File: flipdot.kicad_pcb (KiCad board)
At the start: 2 copper layers, 121.3 x 14.6 mm, 48 parts, among them J1 Conn_01x02_Pin, J2 Conn_01x02_Pin, J3 Conn_01x02_Pin, J4 Conn_01x12_Pin, U5 74HC595

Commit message: split into separate sheets
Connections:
- net /CLK renamed /row1/CLK
- net /DATA_IN renamed /row1/DATA_IN
- net /DATA_OUT renamed /row1/DATA_OUT
- net /LATCH renamed /row1/LATCH
- net /OE* renamed /row1/OE*

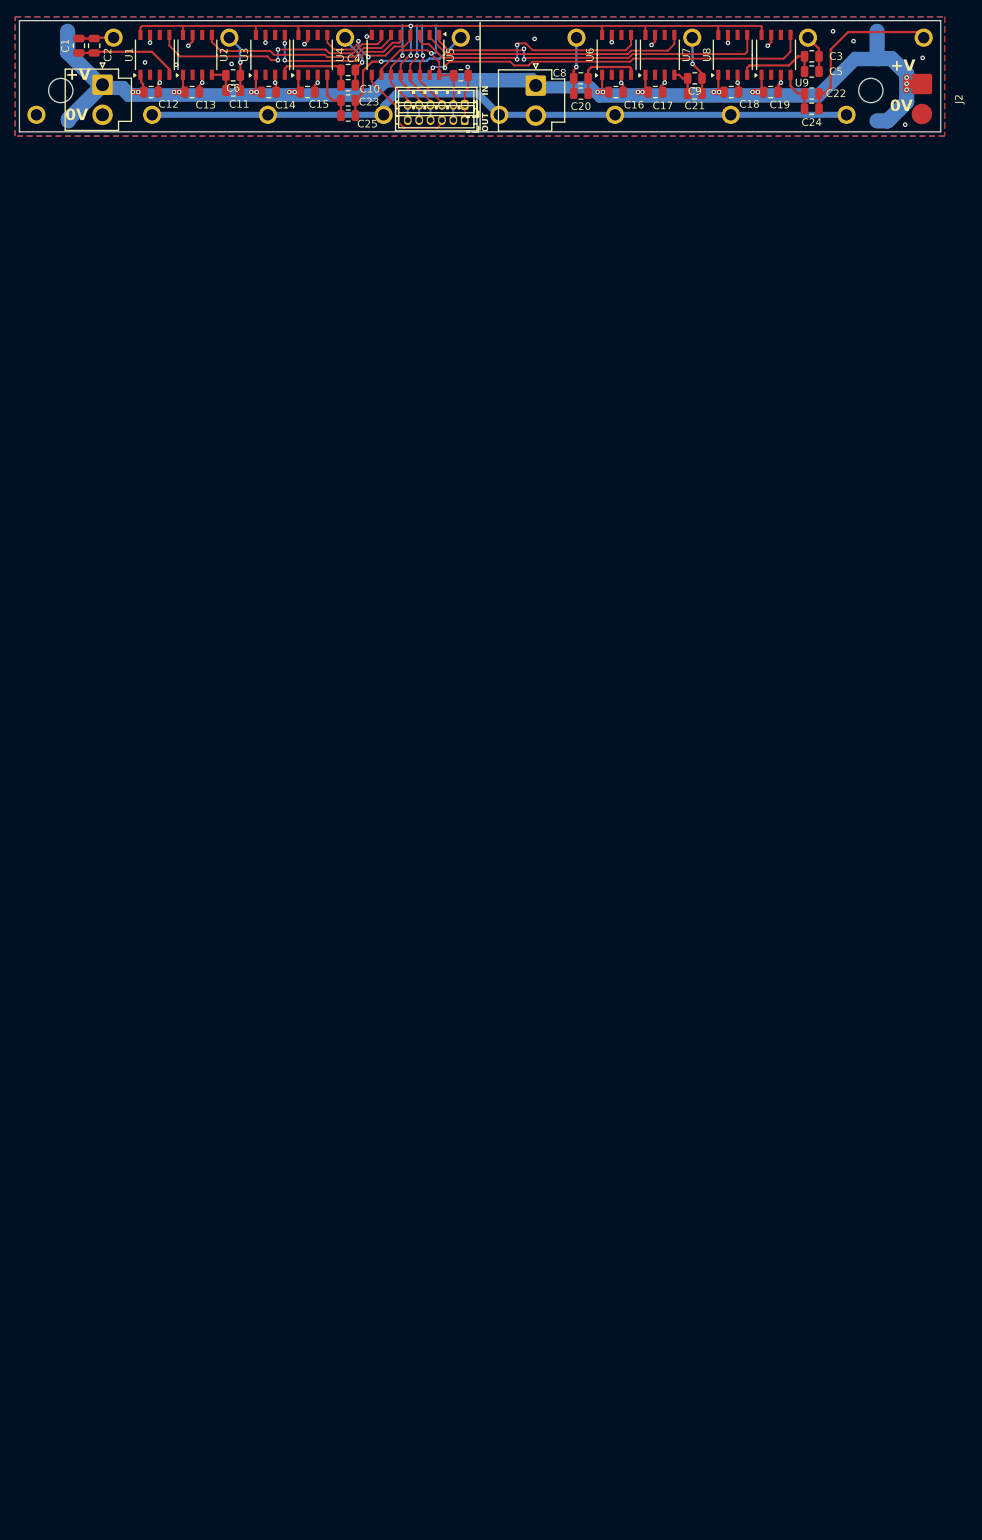
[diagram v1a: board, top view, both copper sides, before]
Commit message: valid 13 row layout
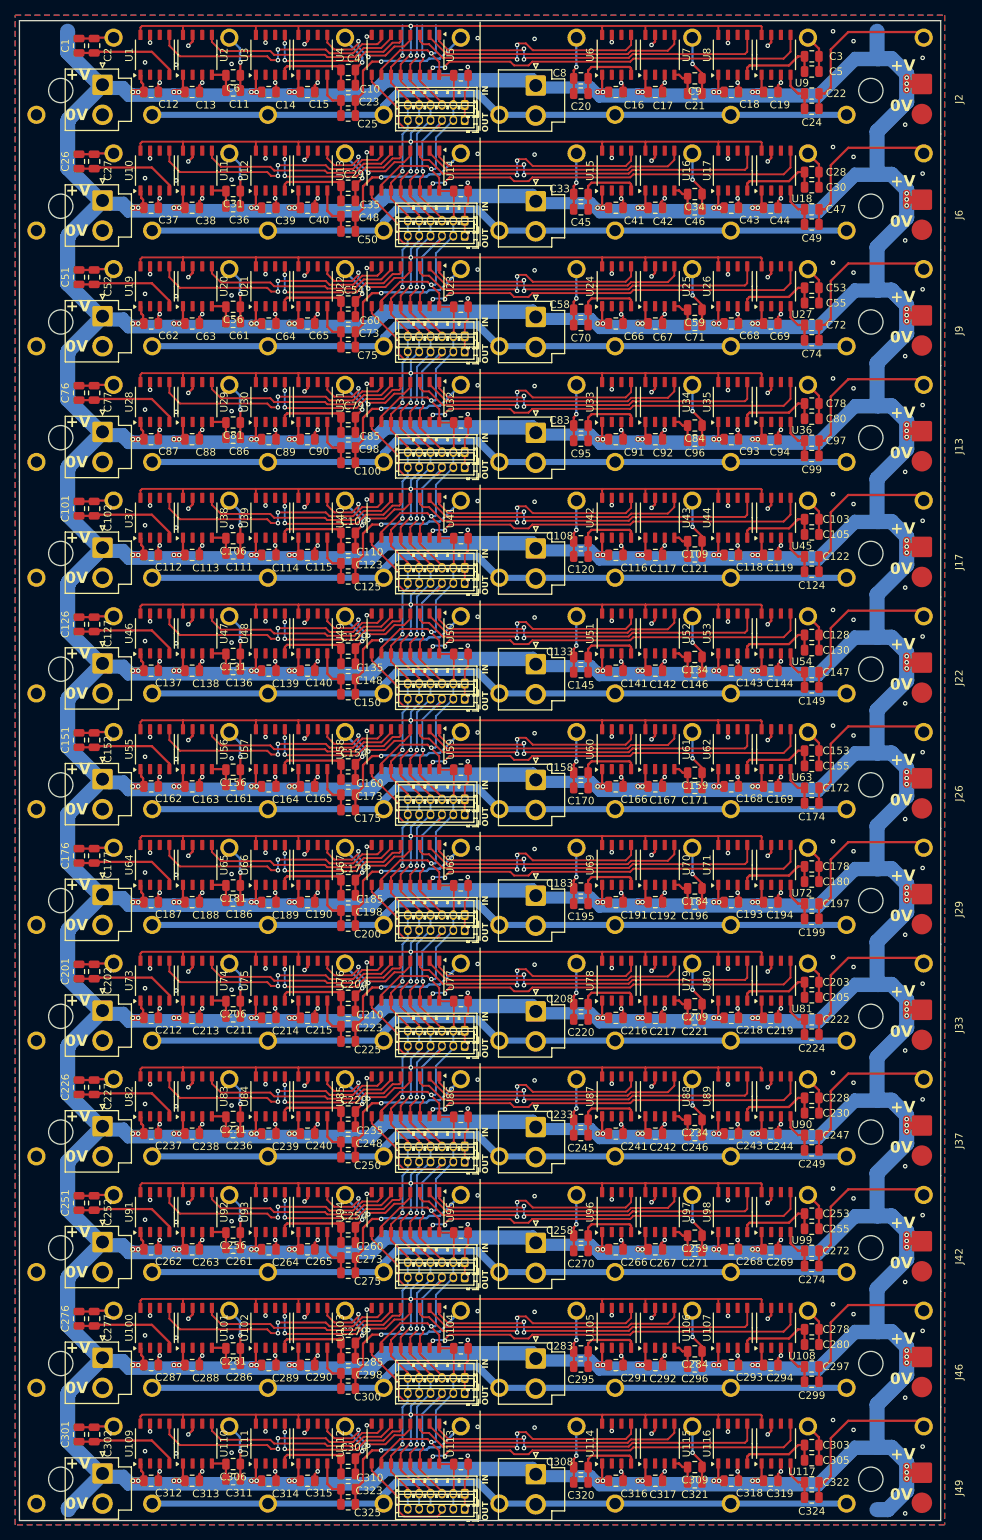
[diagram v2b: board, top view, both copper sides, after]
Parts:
- added C100: 10u, Capacitor_SMD:C_0805_2012Metric, F.Cu at (41.0, 45.8)
- added C101: 10u, Capacitor_SMD:C_0805_2012Metric, F.Cu at (5.60, 51.9)
- added C102: 10u, Capacitor_SMD:C_0805_2012Metric, F.Cu at (7.60, 51.9)
- added C103: 10u, Capacitor_SMD:C_0805_2012Metric, F.Cu at (102.1, 53.3)
- added C104: 10u, Capacitor_SMD:C_0805_2012Metric, F.Cu at (41.0, 55.1)
- added C105: 10u, Capacitor_SMD:C_0805_2012Metric, F.Cu at (102.1, 55.3)
- added C106: 10u, Capacitor_SMD:C_0805_2012Metric, F.Cu at (25.9, 55.8)
- added C107: 10u, Capacitor_SMD:C_0805_2012Metric, F.Cu at (55.9, 55.8)
- added C108: 10u, Capacitor_SMD:C_0805_2012Metric, F.Cu at (71.7, 56.2)
- added C109: 10u, Capacitor_SMD:C_0805_2012Metric, F.Cu at (86.7, 56.2)
- added C110: 10u, Capacitor_SMD:C_0805_2012Metric, F.Cu at (41.0, 57.1)
- added C111: 10u, Capacitor_SMD:C_0805_2012Metric, F.Cu at (25.9, 57.8)
- added C112: 10u, Capacitor_SMD:C_0805_2012Metric, F.Cu at (15.1, 58.0)
- added C113: 10u, Capacitor_SMD:C_0805_2012Metric, F.Cu at (20.5, 58.0)
- added C114: 10u, Capacitor_SMD:C_0805_2012Metric, F.Cu at (30.6, 58.0)
- added C115: 10u, Capacitor_SMD:C_0805_2012Metric, F.Cu at (35.7, 58.0)
- added C116: 10u, Capacitor_SMD:C_0805_2012Metric, F.Cu at (76.3, 58.0)
- added C117: 10u, Capacitor_SMD:C_0805_2012Metric, F.Cu at (81.5, 58.0)
- added C118: 10u, Capacitor_SMD:C_0805_2012Metric, F.Cu at (91.5, 58.0)
- added C119: 10u, Capacitor_SMD:C_0805_2012Metric, F.Cu at (96.7, 58.0)
- added C120: 10u, Capacitor_SMD:C_0805_2012Metric, F.Cu at (71.7, 58.2)
- added C121: 10u, Capacitor_SMD:C_0805_2012Metric, F.Cu at (86.7, 58.2)
- added C122: 10u, Capacitor_SMD:C_0805_2012Metric, F.Cu at (102.1, 58.2)
- added C123: 10u, Capacitor_SMD:C_0805_2012Metric, F.Cu at (41.0, 59.1)
- added C124: 10u, Capacitor_SMD:C_0805_2012Metric, F.Cu at (102.1, 60.2)
- added C125: 10u, Capacitor_SMD:C_0805_2012Metric, F.Cu at (41.0, 61.1)
- added C126: 10u, Capacitor_SMD:C_0805_2012Metric, F.Cu at (5.60, 67.1)
- added C127: 10u, Capacitor_SMD:C_0805_2012Metric, F.Cu at (7.60, 67.1)
- added C128: 10u, Capacitor_SMD:C_0805_2012Metric, F.Cu at (102.1, 68.5)
- added C129: 10u, Capacitor_SMD:C_0805_2012Metric, F.Cu at (41.0, 70.3)
- added C130: 10u, Capacitor_SMD:C_0805_2012Metric, F.Cu at (102.1, 70.5)
- added C131: 10u, Capacitor_SMD:C_0805_2012Metric, F.Cu at (25.9, 71.0)
- added C132: 10u, Capacitor_SMD:C_0805_2012Metric, F.Cu at (55.9, 71.0)
- added C133: 10u, Capacitor_SMD:C_0805_2012Metric, F.Cu at (71.7, 71.4)
- added C134: 10u, Capacitor_SMD:C_0805_2012Metric, F.Cu at (86.7, 71.4)
- added C135: 10u, Capacitor_SMD:C_0805_2012Metric, F.Cu at (41.0, 72.3)
- added C136: 10u, Capacitor_SMD:C_0805_2012Metric, F.Cu at (25.9, 73.0)
- added C137: 10u, Capacitor_SMD:C_0805_2012Metric, F.Cu at (15.1, 73.2)
- added C138: 10u, Capacitor_SMD:C_0805_2012Metric, F.Cu at (20.5, 73.2)
- added C139: 10u, Capacitor_SMD:C_0805_2012Metric, F.Cu at (30.6, 73.2)
- added C140: 10u, Capacitor_SMD:C_0805_2012Metric, F.Cu at (35.7, 73.2)
- added C141: 10u, Capacitor_SMD:C_0805_2012Metric, F.Cu at (76.3, 73.2)
- added C142: 10u, Capacitor_SMD:C_0805_2012Metric, F.Cu at (81.5, 73.2)
- added C143: 10u, Capacitor_SMD:C_0805_2012Metric, F.Cu at (91.5, 73.2)
- added C144: 10u, Capacitor_SMD:C_0805_2012Metric, F.Cu at (96.7, 73.2)
- added C145: 10u, Capacitor_SMD:C_0805_2012Metric, F.Cu at (71.7, 73.4)
- added C146: 10u, Capacitor_SMD:C_0805_2012Metric, F.Cu at (86.7, 73.4)
- added C147: 10u, Capacitor_SMD:C_0805_2012Metric, F.Cu at (102.1, 73.4)
- added C148: 10u, Capacitor_SMD:C_0805_2012Metric, F.Cu at (41.0, 74.3)
- added C149: 10u, Capacitor_SMD:C_0805_2012Metric, F.Cu at (102.1, 75.4)
- added C150: 10u, Capacitor_SMD:C_0805_2012Metric, F.Cu at (41.0, 76.3)
- added C151: 10u, Capacitor_SMD:C_0805_2012Metric, F.Cu at (5.60, 82.3)
- added C152: 10u, Capacitor_SMD:C_0805_2012Metric, F.Cu at (7.60, 82.3)
- added C153: 10u, Capacitor_SMD:C_0805_2012Metric, F.Cu at (102.1, 83.7)
- added C154: 10u, Capacitor_SMD:C_0805_2012Metric, F.Cu at (41.0, 85.5)
- added C155: 10u, Capacitor_SMD:C_0805_2012Metric, F.Cu at (102.1, 85.7)
- added C156: 10u, Capacitor_SMD:C_0805_2012Metric, F.Cu at (25.9, 86.2)
- added C157: 10u, Capacitor_SMD:C_0805_2012Metric, F.Cu at (55.9, 86.2)
- added C158: 10u, Capacitor_SMD:C_0805_2012Metric, F.Cu at (71.7, 86.6)
- added C159: 10u, Capacitor_SMD:C_0805_2012Metric, F.Cu at (86.7, 86.6)
- added C160: 10u, Capacitor_SMD:C_0805_2012Metric, F.Cu at (41.0, 87.5)
- added C161: 10u, Capacitor_SMD:C_0805_2012Metric, F.Cu at (25.9, 88.2)
- added C162: 10u, Capacitor_SMD:C_0805_2012Metric, F.Cu at (15.1, 88.4)
- added C163: 10u, Capacitor_SMD:C_0805_2012Metric, F.Cu at (20.5, 88.4)
- added C164: 10u, Capacitor_SMD:C_0805_2012Metric, F.Cu at (30.6, 88.4)
- added C165: 10u, Capacitor_SMD:C_0805_2012Metric, F.Cu at (35.7, 88.4)
- added C166: 10u, Capacitor_SMD:C_0805_2012Metric, F.Cu at (76.3, 88.4)
- added C167: 10u, Capacitor_SMD:C_0805_2012Metric, F.Cu at (81.5, 88.4)
- added C168: 10u, Capacitor_SMD:C_0805_2012Metric, F.Cu at (91.5, 88.4)
- added C169: 10u, Capacitor_SMD:C_0805_2012Metric, F.Cu at (96.7, 88.4)
- added C170: 10u, Capacitor_SMD:C_0805_2012Metric, F.Cu at (71.7, 88.6)
- added C171: 10u, Capacitor_SMD:C_0805_2012Metric, F.Cu at (86.7, 88.6)
- added C172: 10u, Capacitor_SMD:C_0805_2012Metric, F.Cu at (102.1, 88.6)
- added C173: 10u, Capacitor_SMD:C_0805_2012Metric, F.Cu at (41.0, 89.5)
- added C174: 10u, Capacitor_SMD:C_0805_2012Metric, F.Cu at (102.1, 90.6)
- added C175: 10u, Capacitor_SMD:C_0805_2012Metric, F.Cu at (41.0, 91.5)
- added C176: 10u, Capacitor_SMD:C_0805_2012Metric, F.Cu at (5.60, 97.6)
- added C177: 10u, Capacitor_SMD:C_0805_2012Metric, F.Cu at (7.60, 97.6)
- added C178: 10u, Capacitor_SMD:C_0805_2012Metric, F.Cu at (102.1, 99.0)
- added C179: 10u, Capacitor_SMD:C_0805_2012Metric, F.Cu at (41.0, 100.8)
- added C180: 10u, Capacitor_SMD:C_0805_2012Metric, F.Cu at (102.1, 101.0)
- added C181: 10u, Capacitor_SMD:C_0805_2012Metric, F.Cu at (25.9, 101.5)
- added C182: 10u, Capacitor_SMD:C_0805_2012Metric, F.Cu at (55.9, 101.5)
- added C183: 10u, Capacitor_SMD:C_0805_2012Metric, F.Cu at (71.7, 101.9)
- added C184: 10u, Capacitor_SMD:C_0805_2012Metric, F.Cu at (86.7, 101.9)
- added C185: 10u, Capacitor_SMD:C_0805_2012Metric, F.Cu at (41.0, 102.8)
- added C186: 10u, Capacitor_SMD:C_0805_2012Metric, F.Cu at (25.9, 103.5)
- added C187: 10u, Capacitor_SMD:C_0805_2012Metric, F.Cu at (15.1, 103.7)
- added C188: 10u, Capacitor_SMD:C_0805_2012Metric, F.Cu at (20.5, 103.7)
- added C189: 10u, Capacitor_SMD:C_0805_2012Metric, F.Cu at (30.6, 103.7)
- added C190: 10u, Capacitor_SMD:C_0805_2012Metric, F.Cu at (35.7, 103.7)
- added C191: 10u, Capacitor_SMD:C_0805_2012Metric, F.Cu at (76.3, 103.7)
- added C192: 10u, Capacitor_SMD:C_0805_2012Metric, F.Cu at (81.5, 103.7)
- added C193: 10u, Capacitor_SMD:C_0805_2012Metric, F.Cu at (91.5, 103.7)
- added C194: 10u, Capacitor_SMD:C_0805_2012Metric, F.Cu at (96.7, 103.7)
- added C195: 10u, Capacitor_SMD:C_0805_2012Metric, F.Cu at (71.7, 103.9)
- added C196: 10u, Capacitor_SMD:C_0805_2012Metric, F.Cu at (86.7, 103.9)
- added C197: 10u, Capacitor_SMD:C_0805_2012Metric, F.Cu at (102.1, 103.9)
- added C198: 10u, Capacitor_SMD:C_0805_2012Metric, F.Cu at (41.0, 104.8)
- added C199: 10u, Capacitor_SMD:C_0805_2012Metric, F.Cu at (102.1, 105.9)
- added C200: 10u, Capacitor_SMD:C_0805_2012Metric, F.Cu at (41.0, 106.8)
- added C201: 10u, Capacitor_SMD:C_0805_2012Metric, F.Cu at (5.60, 112.8)
- added C202: 10u, Capacitor_SMD:C_0805_2012Metric, F.Cu at (7.60, 112.8)
- added C203: 10u, Capacitor_SMD:C_0805_2012Metric, F.Cu at (102.1, 114.2)
- added C204: 10u, Capacitor_SMD:C_0805_2012Metric, F.Cu at (41.0, 116.0)
- added C205: 10u, Capacitor_SMD:C_0805_2012Metric, F.Cu at (102.1, 116.2)
- added C206: 10u, Capacitor_SMD:C_0805_2012Metric, F.Cu at (25.9, 116.7)
- added C207: 10u, Capacitor_SMD:C_0805_2012Metric, F.Cu at (55.9, 116.7)
- added C208: 10u, Capacitor_SMD:C_0805_2012Metric, F.Cu at (71.7, 117.1)
- added C209: 10u, Capacitor_SMD:C_0805_2012Metric, F.Cu at (86.7, 117.1)
- added C210: 10u, Capacitor_SMD:C_0805_2012Metric, F.Cu at (41.0, 118.0)
- added C211: 10u, Capacitor_SMD:C_0805_2012Metric, F.Cu at (25.9, 118.7)
- added C212: 10u, Capacitor_SMD:C_0805_2012Metric, F.Cu at (15.1, 118.9)
- added C213: 10u, Capacitor_SMD:C_0805_2012Metric, F.Cu at (20.5, 118.9)
- added C214: 10u, Capacitor_SMD:C_0805_2012Metric, F.Cu at (30.6, 118.9)
- added C215: 10u, Capacitor_SMD:C_0805_2012Metric, F.Cu at (35.7, 118.9)
- added C216: 10u, Capacitor_SMD:C_0805_2012Metric, F.Cu at (76.3, 118.9)
- added C217: 10u, Capacitor_SMD:C_0805_2012Metric, F.Cu at (81.5, 118.9)
- added C218: 10u, Capacitor_SMD:C_0805_2012Metric, F.Cu at (91.5, 118.9)
- added C219: 10u, Capacitor_SMD:C_0805_2012Metric, F.Cu at (96.7, 118.9)
- added C220: 10u, Capacitor_SMD:C_0805_2012Metric, F.Cu at (71.7, 119.1)
- added C221: 10u, Capacitor_SMD:C_0805_2012Metric, F.Cu at (86.7, 119.1)
- added C222: 10u, Capacitor_SMD:C_0805_2012Metric, F.Cu at (102.1, 119.1)
- added C223: 10u, Capacitor_SMD:C_0805_2012Metric, F.Cu at (41.0, 120.0)
- added C224: 10u, Capacitor_SMD:C_0805_2012Metric, F.Cu at (102.1, 121.1)
- added C225: 10u, Capacitor_SMD:C_0805_2012Metric, F.Cu at (41.0, 122.0)
- added C226: 10u, Capacitor_SMD:C_0805_2012Metric, F.Cu at (5.60, 128.1)
- added C227: 10u, Capacitor_SMD:C_0805_2012Metric, F.Cu at (7.60, 128.1)
- added C228: 10u, Capacitor_SMD:C_0805_2012Metric, F.Cu at (102.1, 129.5)
- added C229: 10u, Capacitor_SMD:C_0805_2012Metric, F.Cu at (41.0, 131.3)
- added C230: 10u, Capacitor_SMD:C_0805_2012Metric, F.Cu at (102.1, 131.5)
- added C231: 10u, Capacitor_SMD:C_0805_2012Metric, F.Cu at (25.9, 132.0)
- added C232: 10u, Capacitor_SMD:C_0805_2012Metric, F.Cu at (55.9, 132.0)
- added C233: 10u, Capacitor_SMD:C_0805_2012Metric, F.Cu at (71.7, 132.4)
- added C234: 10u, Capacitor_SMD:C_0805_2012Metric, F.Cu at (86.7, 132.4)
- added C235: 10u, Capacitor_SMD:C_0805_2012Metric, F.Cu at (41.0, 133.3)
- added C236: 10u, Capacitor_SMD:C_0805_2012Metric, F.Cu at (25.9, 134.0)
- added C237: 10u, Capacitor_SMD:C_0805_2012Metric, F.Cu at (15.1, 134.2)
- added C238: 10u, Capacitor_SMD:C_0805_2012Metric, F.Cu at (20.5, 134.2)
- added C239: 10u, Capacitor_SMD:C_0805_2012Metric, F.Cu at (30.6, 134.2)
- added C240: 10u, Capacitor_SMD:C_0805_2012Metric, F.Cu at (35.7, 134.2)
- added C241: 10u, Capacitor_SMD:C_0805_2012Metric, F.Cu at (76.3, 134.2)
- added C242: 10u, Capacitor_SMD:C_0805_2012Metric, F.Cu at (81.5, 134.2)
- added C243: 10u, Capacitor_SMD:C_0805_2012Metric, F.Cu at (91.5, 134.2)
- added C244: 10u, Capacitor_SMD:C_0805_2012Metric, F.Cu at (96.7, 134.2)
- added C245: 10u, Capacitor_SMD:C_0805_2012Metric, F.Cu at (71.7, 134.4)
- added C246: 10u, Capacitor_SMD:C_0805_2012Metric, F.Cu at (86.7, 134.4)
- added C247: 10u, Capacitor_SMD:C_0805_2012Metric, F.Cu at (102.1, 134.4)
- added C248: 10u, Capacitor_SMD:C_0805_2012Metric, F.Cu at (41.0, 135.3)
- added C249: 10u, Capacitor_SMD:C_0805_2012Metric, F.Cu at (102.1, 136.4)
- added C250: 10u, Capacitor_SMD:C_0805_2012Metric, F.Cu at (41.0, 137.3)
- added C251: 10u, Capacitor_SMD:C_0805_2012Metric, F.Cu at (5.60, 143.3)
- added C252: 10u, Capacitor_SMD:C_0805_2012Metric, F.Cu at (7.60, 143.3)
- added C253: 10u, Capacitor_SMD:C_0805_2012Metric, F.Cu at (102.1, 144.7)
- added C254: 10u, Capacitor_SMD:C_0805_2012Metric, F.Cu at (41.0, 146.5)
- added C255: 10u, Capacitor_SMD:C_0805_2012Metric, F.Cu at (102.1, 146.7)
- added C256: 10u, Capacitor_SMD:C_0805_2012Metric, F.Cu at (25.9, 147.2)
- added C257: 10u, Capacitor_SMD:C_0805_2012Metric, F.Cu at (55.9, 147.2)
- added C258: 10u, Capacitor_SMD:C_0805_2012Metric, F.Cu at (71.7, 147.6)
- added C259: 10u, Capacitor_SMD:C_0805_2012Metric, F.Cu at (86.7, 147.6)
- added C26: 10u, Capacitor_SMD:C_0805_2012Metric, F.Cu at (5.60, 6.14)
- added C260: 10u, Capacitor_SMD:C_0805_2012Metric, F.Cu at (41.0, 148.5)
- added C261: 10u, Capacitor_SMD:C_0805_2012Metric, F.Cu at (25.9, 149.2)
- added C262: 10u, Capacitor_SMD:C_0805_2012Metric, F.Cu at (15.1, 149.4)
- added C263: 10u, Capacitor_SMD:C_0805_2012Metric, F.Cu at (20.5, 149.4)
- added C264: 10u, Capacitor_SMD:C_0805_2012Metric, F.Cu at (30.6, 149.4)
- added C265: 10u, Capacitor_SMD:C_0805_2012Metric, F.Cu at (35.7, 149.4)
- added C266: 10u, Capacitor_SMD:C_0805_2012Metric, F.Cu at (76.3, 149.4)
- added C267: 10u, Capacitor_SMD:C_0805_2012Metric, F.Cu at (81.5, 149.4)
- added C268: 10u, Capacitor_SMD:C_0805_2012Metric, F.Cu at (91.5, 149.4)
- added C269: 10u, Capacitor_SMD:C_0805_2012Metric, F.Cu at (96.7, 149.4)
- added C27: 10u, Capacitor_SMD:C_0805_2012Metric, F.Cu at (7.60, 6.14)
- added C270: 10u, Capacitor_SMD:C_0805_2012Metric, F.Cu at (71.7, 149.6)
- added C271: 10u, Capacitor_SMD:C_0805_2012Metric, F.Cu at (86.7, 149.6)
- added C272: 10u, Capacitor_SMD:C_0805_2012Metric, F.Cu at (102.1, 149.6)
- added C273: 10u, Capacitor_SMD:C_0805_2012Metric, F.Cu at (41.0, 150.5)
- added C274: 10u, Capacitor_SMD:C_0805_2012Metric, F.Cu at (102.1, 151.6)
- added C275: 10u, Capacitor_SMD:C_0805_2012Metric, F.Cu at (41.0, 152.5)
- added C276: 10u, Capacitor_SMD:C_0805_2012Metric, F.Cu at (5.60, 158.5)
- added C277: 10u, Capacitor_SMD:C_0805_2012Metric, F.Cu at (7.60, 158.5)
- added C278: 10u, Capacitor_SMD:C_0805_2012Metric, F.Cu at (102.1, 159.9)
- added C279: 10u, Capacitor_SMD:C_0805_2012Metric, F.Cu at (41.0, 161.7)
- added C28: 10u, Capacitor_SMD:C_0805_2012Metric, F.Cu at (102.1, 7.54)
- added C280: 10u, Capacitor_SMD:C_0805_2012Metric, F.Cu at (102.1, 161.9)
- added C281: 10u, Capacitor_SMD:C_0805_2012Metric, F.Cu at (25.9, 162.4)
- added C282: 10u, Capacitor_SMD:C_0805_2012Metric, F.Cu at (55.9, 162.4)
- added C283: 10u, Capacitor_SMD:C_0805_2012Metric, F.Cu at (71.7, 162.8)
- added C284: 10u, Capacitor_SMD:C_0805_2012Metric, F.Cu at (86.7, 162.8)
- added C285: 10u, Capacitor_SMD:C_0805_2012Metric, F.Cu at (41.0, 163.7)
- added C286: 10u, Capacitor_SMD:C_0805_2012Metric, F.Cu at (25.9, 164.4)
- added C287: 10u, Capacitor_SMD:C_0805_2012Metric, F.Cu at (15.1, 164.6)
- added C288: 10u, Capacitor_SMD:C_0805_2012Metric, F.Cu at (20.5, 164.6)
- added C289: 10u, Capacitor_SMD:C_0805_2012Metric, F.Cu at (30.6, 164.6)
- added C29: 10u, Capacitor_SMD:C_0805_2012Metric, F.Cu at (41.0, 9.34)
- added C290: 10u, Capacitor_SMD:C_0805_2012Metric, F.Cu at (35.7, 164.6)
- added C291: 10u, Capacitor_SMD:C_0805_2012Metric, F.Cu at (76.3, 164.6)
- added C292: 10u, Capacitor_SMD:C_0805_2012Metric, F.Cu at (81.5, 164.6)
- added C293: 10u, Capacitor_SMD:C_0805_2012Metric, F.Cu at (91.5, 164.6)
- added C294: 10u, Capacitor_SMD:C_0805_2012Metric, F.Cu at (96.7, 164.6)
- added C295: 10u, Capacitor_SMD:C_0805_2012Metric, F.Cu at (71.7, 164.8)
- added C296: 10u, Capacitor_SMD:C_0805_2012Metric, F.Cu at (86.7, 164.8)
- added C297: 10u, Capacitor_SMD:C_0805_2012Metric, F.Cu at (102.1, 164.8)
- added C298: 10u, Capacitor_SMD:C_0805_2012Metric, F.Cu at (41.0, 165.7)
- added C299: 10u, Capacitor_SMD:C_0805_2012Metric, F.Cu at (102.1, 166.8)
- added C30: 10u, Capacitor_SMD:C_0805_2012Metric, F.Cu at (102.1, 9.54)
- added C300: 10u, Capacitor_SMD:C_0805_2012Metric, F.Cu at (41.0, 167.7)
- added C301: 10u, Capacitor_SMD:C_0805_2012Metric, F.Cu at (5.60, 173.8)
- added C302: 10u, Capacitor_SMD:C_0805_2012Metric, F.Cu at (7.60, 173.8)
- added C303: 10u, Capacitor_SMD:C_0805_2012Metric, F.Cu at (102.1, 175.2)
- added C304: 10u, Capacitor_SMD:C_0805_2012Metric, F.Cu at (41.0, 177.0)
- added C305: 10u, Capacitor_SMD:C_0805_2012Metric, F.Cu at (102.1, 177.2)
- added C306: 10u, Capacitor_SMD:C_0805_2012Metric, F.Cu at (25.9, 177.7)
- added C307: 10u, Capacitor_SMD:C_0805_2012Metric, F.Cu at (55.9, 177.7)
- added C308: 10u, Capacitor_SMD:C_0805_2012Metric, F.Cu at (71.7, 178.1)
- added C309: 10u, Capacitor_SMD:C_0805_2012Metric, F.Cu at (86.7, 178.1)
- added C31: 10u, Capacitor_SMD:C_0805_2012Metric, F.Cu at (25.9, 10.0)
- added C310: 10u, Capacitor_SMD:C_0805_2012Metric, F.Cu at (41.0, 179.0)
- added C311: 10u, Capacitor_SMD:C_0805_2012Metric, F.Cu at (25.9, 179.7)
- added C312: 10u, Capacitor_SMD:C_0805_2012Metric, F.Cu at (15.1, 179.9)
- added C313: 10u, Capacitor_SMD:C_0805_2012Metric, F.Cu at (20.5, 179.9)
- added C314: 10u, Capacitor_SMD:C_0805_2012Metric, F.Cu at (30.6, 179.9)
- added C315: 10u, Capacitor_SMD:C_0805_2012Metric, F.Cu at (35.7, 179.9)
- added C316: 10u, Capacitor_SMD:C_0805_2012Metric, F.Cu at (76.3, 179.9)
- added C317: 10u, Capacitor_SMD:C_0805_2012Metric, F.Cu at (81.5, 179.9)
- added C318: 10u, Capacitor_SMD:C_0805_2012Metric, F.Cu at (91.5, 179.9)
- added C319: 10u, Capacitor_SMD:C_0805_2012Metric, F.Cu at (96.7, 179.9)
- added C32: 10u, Capacitor_SMD:C_0805_2012Metric, F.Cu at (55.9, 10.0)
- added C320: 10u, Capacitor_SMD:C_0805_2012Metric, F.Cu at (71.7, 180.1)
- added C321: 10u, Capacitor_SMD:C_0805_2012Metric, F.Cu at (86.7, 180.1)
- added C322: 10u, Capacitor_SMD:C_0805_2012Metric, F.Cu at (102.1, 180.1)
- added C323: 10u, Capacitor_SMD:C_0805_2012Metric, F.Cu at (41.0, 181.0)
- added C324: 10u, Capacitor_SMD:C_0805_2012Metric, F.Cu at (102.1, 182.1)
- added C325: 10u, Capacitor_SMD:C_0805_2012Metric, F.Cu at (41.0, 183.0)
- added C33: 10u, Capacitor_SMD:C_0805_2012Metric, F.Cu at (71.7, 10.4)
- added C34: 10u, Capacitor_SMD:C_0805_2012Metric, F.Cu at (86.7, 10.4)
- added C35: 10u, Capacitor_SMD:C_0805_2012Metric, F.Cu at (41.0, 11.3)
- added C36: 10u, Capacitor_SMD:C_0805_2012Metric, F.Cu at (25.9, 12.0)
- added C37: 10u, Capacitor_SMD:C_0805_2012Metric, F.Cu at (15.1, 12.2)
- added C38: 10u, Capacitor_SMD:C_0805_2012Metric, F.Cu at (20.5, 12.2)
- added C39: 10u, Capacitor_SMD:C_0805_2012Metric, F.Cu at (30.6, 12.2)
- added C40: 10u, Capacitor_SMD:C_0805_2012Metric, F.Cu at (35.7, 12.2)
- added C41: 10u, Capacitor_SMD:C_0805_2012Metric, F.Cu at (76.3, 12.2)
- added C42: 10u, Capacitor_SMD:C_0805_2012Metric, F.Cu at (81.5, 12.2)
- added C43: 10u, Capacitor_SMD:C_0805_2012Metric, F.Cu at (91.5, 12.2)
- added C44: 10u, Capacitor_SMD:C_0805_2012Metric, F.Cu at (96.7, 12.2)
- added C45: 10u, Capacitor_SMD:C_0805_2012Metric, F.Cu at (71.7, 12.4)
- added C46: 10u, Capacitor_SMD:C_0805_2012Metric, F.Cu at (86.7, 12.4)
- added C47: 10u, Capacitor_SMD:C_0805_2012Metric, F.Cu at (102.1, 12.4)
- added C48: 10u, Capacitor_SMD:C_0805_2012Metric, F.Cu at (41.0, 13.3)
- added C49: 10u, Capacitor_SMD:C_0805_2012Metric, F.Cu at (102.1, 14.4)
- added C50: 10u, Capacitor_SMD:C_0805_2012Metric, F.Cu at (41.0, 15.3)
- added C51: 10u, Capacitor_SMD:C_0805_2012Metric, F.Cu at (5.60, 21.4)
- added C52: 10u, Capacitor_SMD:C_0805_2012Metric, F.Cu at (7.60, 21.4)
- added C53: 10u, Capacitor_SMD:C_0805_2012Metric, F.Cu at (102.1, 22.8)
- added C54: 10u, Capacitor_SMD:C_0805_2012Metric, F.Cu at (41.0, 24.6)
- added C55: 10u, Capacitor_SMD:C_0805_2012Metric, F.Cu at (102.1, 24.8)
- added C56: 10u, Capacitor_SMD:C_0805_2012Metric, F.Cu at (25.9, 25.3)
- added C57: 10u, Capacitor_SMD:C_0805_2012Metric, F.Cu at (55.9, 25.3)
- added C58: 10u, Capacitor_SMD:C_0805_2012Metric, F.Cu at (71.7, 25.7)
- added C59: 10u, Capacitor_SMD:C_0805_2012Metric, F.Cu at (86.7, 25.7)
- added C60: 10u, Capacitor_SMD:C_0805_2012Metric, F.Cu at (41.0, 26.6)
- added C61: 10u, Capacitor_SMD:C_0805_2012Metric, F.Cu at (25.9, 27.3)
- added C62: 10u, Capacitor_SMD:C_0805_2012Metric, F.Cu at (15.1, 27.5)
- added C63: 10u, Capacitor_SMD:C_0805_2012Metric, F.Cu at (20.5, 27.5)
- added C64: 10u, Capacitor_SMD:C_0805_2012Metric, F.Cu at (30.6, 27.5)
- added C65: 10u, Capacitor_SMD:C_0805_2012Metric, F.Cu at (35.7, 27.5)
- added C66: 10u, Capacitor_SMD:C_0805_2012Metric, F.Cu at (76.3, 27.5)
- added C67: 10u, Capacitor_SMD:C_0805_2012Metric, F.Cu at (81.5, 27.5)
- added C68: 10u, Capacitor_SMD:C_0805_2012Metric, F.Cu at (91.5, 27.5)
- added C69: 10u, Capacitor_SMD:C_0805_2012Metric, F.Cu at (96.7, 27.5)
- added C70: 10u, Capacitor_SMD:C_0805_2012Metric, F.Cu at (71.7, 27.7)
- added C71: 10u, Capacitor_SMD:C_0805_2012Metric, F.Cu at (86.7, 27.7)
- added C72: 10u, Capacitor_SMD:C_0805_2012Metric, F.Cu at (102.1, 27.7)
- added C73: 10u, Capacitor_SMD:C_0805_2012Metric, F.Cu at (41.0, 28.6)
- added C74: 10u, Capacitor_SMD:C_0805_2012Metric, F.Cu at (102.1, 29.7)
- added C75: 10u, Capacitor_SMD:C_0805_2012Metric, F.Cu at (41.0, 30.6)
- added C76: 10u, Capacitor_SMD:C_0805_2012Metric, F.Cu at (5.60, 36.6)
- added C77: 10u, Capacitor_SMD:C_0805_2012Metric, F.Cu at (7.60, 36.6)
- added C78: 10u, Capacitor_SMD:C_0805_2012Metric, F.Cu at (102.1, 38.0)
- added C79: 10u, Capacitor_SMD:C_0805_2012Metric, F.Cu at (41.0, 39.8)
- added C80: 10u, Capacitor_SMD:C_0805_2012Metric, F.Cu at (102.1, 40.0)
- added C81: 10u, Capacitor_SMD:C_0805_2012Metric, F.Cu at (25.9, 40.5)
- added C82: 10u, Capacitor_SMD:C_0805_2012Metric, F.Cu at (55.9, 40.5)
- added C83: 10u, Capacitor_SMD:C_0805_2012Metric, F.Cu at (71.7, 40.9)
- added C84: 10u, Capacitor_SMD:C_0805_2012Metric, F.Cu at (86.7, 40.9)
- added C85: 10u, Capacitor_SMD:C_0805_2012Metric, F.Cu at (41.0, 41.8)
- added C86: 10u, Capacitor_SMD:C_0805_2012Metric, F.Cu at (25.9, 42.5)
- added C87: 10u, Capacitor_SMD:C_0805_2012Metric, F.Cu at (15.1, 42.7)
- added C88: 10u, Capacitor_SMD:C_0805_2012Metric, F.Cu at (20.5, 42.7)
- added C89: 10u, Capacitor_SMD:C_0805_2012Metric, F.Cu at (30.6, 42.7)
- added C90: 10u, Capacitor_SMD:C_0805_2012Metric, F.Cu at (35.7, 42.7)
- added C91: 10u, Capacitor_SMD:C_0805_2012Metric, F.Cu at (76.3, 42.7)
- added C92: 10u, Capacitor_SMD:C_0805_2012Metric, F.Cu at (81.5, 42.7)
- added C93: 10u, Capacitor_SMD:C_0805_2012Metric, F.Cu at (91.5, 42.7)
- added C94: 10u, Capacitor_SMD:C_0805_2012Metric, F.Cu at (96.7, 42.7)
- added C95: 10u, Capacitor_SMD:C_0805_2012Metric, F.Cu at (71.7, 42.9)
- added C96: 10u, Capacitor_SMD:C_0805_2012Metric, F.Cu at (86.7, 42.9)
- added C97: 10u, Capacitor_SMD:C_0805_2012Metric, F.Cu at (102.1, 42.9)
- added C98: 10u, Capacitor_SMD:C_0805_2012Metric, F.Cu at (41.0, 43.8)
- added C99: 10u, Capacitor_SMD:C_0805_2012Metric, F.Cu at (102.1, 44.9)
- added H10: MountingHole, MountingHole:MountingHole_3.2mm_M3_DIN965, F.Cu at (109.9, 57.8)
- added H11: MountingHole, MountingHole:MountingHole_3.2mm_M3_DIN965, F.Cu at (3.20, 73.0)
- added H12: MountingHole, MountingHole:MountingHole_3.2mm_M3_DIN965, F.Cu at (109.9, 73.0)
- added H13: MountingHole, MountingHole:MountingHole_3.2mm_M3_DIN965, F.Cu at (3.20, 88.2)
- added H14: MountingHole, MountingHole:MountingHole_3.2mm_M3_DIN965, F.Cu at (109.9, 88.2)
- added H15: MountingHole, MountingHole:MountingHole_3.2mm_M3_DIN965, F.Cu at (3.20, 103.5)
- added H16: MountingHole, MountingHole:MountingHole_3.2mm_M3_DIN965, F.Cu at (109.9, 103.5)
- added H17: MountingHole, MountingHole:MountingHole_3.2mm_M3_DIN965, F.Cu at (3.20, 118.7)
- added H18: MountingHole, MountingHole:MountingHole_3.2mm_M3_DIN965, F.Cu at (109.9, 118.7)
- added H19: MountingHole, MountingHole:MountingHole_3.2mm_M3_DIN965, F.Cu at (3.20, 134.0)
- added H20: MountingHole, MountingHole:MountingHole_3.2mm_M3_DIN965, F.Cu at (109.9, 134.0)
- added H21: MountingHole, MountingHole:MountingHole_3.2mm_M3_DIN965, F.Cu at (3.20, 149.2)
- added H22: MountingHole, MountingHole:MountingHole_3.2mm_M3_DIN965, F.Cu at (109.9, 149.2)
- added H23: MountingHole, MountingHole:MountingHole_3.2mm_M3_DIN965, F.Cu at (3.20, 164.4)
- added H24: MountingHole, MountingHole:MountingHole_3.2mm_M3_DIN965, F.Cu at (109.9, 164.4)
- added H25: MountingHole, MountingHole:MountingHole_3.2mm_M3_DIN965, F.Cu at (3.20, 179.7)
- added H26: MountingHole, MountingHole:MountingHole_3.2mm_M3_DIN965, F.Cu at (109.9, 179.7)
- added H3: MountingHole, MountingHole:MountingHole_3.2mm_M3_DIN965, F.Cu at (3.20, 12.0)
- added H4: MountingHole, MountingHole:MountingHole_3.2mm_M3_DIN965, F.Cu at (109.9, 12.0)
- added H5: MountingHole, MountingHole:MountingHole_3.2mm_M3_DIN965, F.Cu at (3.20, 27.3)
- added H6: MountingHole, MountingHole:MountingHole_3.2mm_M3_DIN965, F.Cu at (109.9, 27.3)
- added H7: MountingHole, MountingHole:MountingHole_3.2mm_M3_DIN965, F.Cu at (3.20, 42.5)
- added H8: MountingHole, MountingHole:MountingHole_3.2mm_M3_DIN965, F.Cu at (109.9, 42.5)
- added H9: MountingHole, MountingHole:MountingHole_3.2mm_M3_DIN965, F.Cu at (3.20, 57.8)
- added J10: Conn_01x02_Pin, Connector_JST:JST_VH_B2P-VH_1x02_P3.96mm_Vertical, F.Cu at (8.70, 26.5)
- added J11: Conn_01x02_Pin, Connector_JST:JST_VH_B2P-VH_1x02_P3.96mm_Vertical, F.Cu at (65.8, 26.6)
- added J12: Conn_01x12_Pin, Connector_JST:JST_ZH_B6B-ZR_1x06_P1.50mm_Vertical, F.Cu at (56.4, 31.2)
- added J13: Conn_01x02_Pin, Connector_JST:JST_VH_B2P-VH_1x02_P3.96mm_Vertical, F.Cu at (116.6, 41.7)
- added J14: Conn_01x02_Pin, Connector_JST:JST_VH_B2P-VH_1x02_P3.96mm_Vertical, F.Cu at (8.70, 41.8)
- added J15: Conn_01x02_Pin, Connector_JST:JST_VH_B2P-VH_1x02_P3.96mm_Vertical, F.Cu at (65.8, 41.9)
- added J16: Conn_01x12_Pin, Connector_JST:JST_ZH_B6B-ZR_1x06_P1.50mm_Vertical, F.Cu at (56.4, 46.4)
- added J17: Conn_01x02_Pin, Connector_JST:JST_VH_B2P-VH_1x02_P3.96mm_Vertical, F.Cu at (116.6, 56.9)
- added J18: Conn_01x02_Pin, Connector_JST:JST_VH_B2P-VH_1x02_P3.96mm_Vertical, F.Cu at (8.70, 57.0)
- added J19: Conn_01x02_Pin, Connector_JST:JST_VH_B2P-VH_1x02_P3.96mm_Vertical, F.Cu at (65.8, 57.1)
- added J20: Conn_01x12_Pin, Connector_JST:JST_ZH_B6B-ZR_1x06_P1.50mm_Vertical, F.Cu at (56.4, 61.7)
- added J21: Conn_01x02_Pin, Connector_JST:JST_VH_B2P-VH_1x02_P3.96mm_Vertical, F.Cu at (8.70, 72.2)
- added J22: Conn_01x02_Pin, Connector_JST:JST_VH_B2P-VH_1x02_P3.96mm_Vertical, F.Cu at (116.6, 72.1)
- added J23: Conn_01x02_Pin, Connector_JST:JST_VH_B2P-VH_1x02_P3.96mm_Vertical, F.Cu at (65.8, 72.3)
- added J24: Conn_01x12_Pin, Connector_JST:JST_ZH_B6B-ZR_1x06_P1.50mm_Vertical, F.Cu at (56.4, 76.9)
- added J25: Conn_01x02_Pin, Connector_JST:JST_VH_B2P-VH_1x02_P3.96mm_Vertical, F.Cu at (8.70, 87.5)
- added J26: Conn_01x02_Pin, Connector_JST:JST_VH_B2P-VH_1x02_P3.96mm_Vertical, F.Cu at (116.6, 87.4)
- added J27: Conn_01x02_Pin, Connector_JST:JST_VH_B2P-VH_1x02_P3.96mm_Vertical, F.Cu at (65.8, 87.6)
- added J28: Conn_01x12_Pin, Connector_JST:JST_ZH_B6B-ZR_1x06_P1.50mm_Vertical, F.Cu at (56.4, 92.1)
- added J29: Conn_01x02_Pin, Connector_JST:JST_VH_B2P-VH_1x02_P3.96mm_Vertical, F.Cu at (116.6, 102.6)
- added J30: Conn_01x02_Pin, Connector_JST:JST_VH_B2P-VH_1x02_P3.96mm_Vertical, F.Cu at (8.70, 102.7)
- added J31: Conn_01x02_Pin, Connector_JST:JST_VH_B2P-VH_1x02_P3.96mm_Vertical, F.Cu at (65.8, 102.8)
- added J32: Conn_01x12_Pin, Connector_JST:JST_ZH_B6B-ZR_1x06_P1.50mm_Vertical, F.Cu at (56.4, 107.4)
- added J33: Conn_01x02_Pin, Connector_JST:JST_VH_B2P-VH_1x02_P3.96mm_Vertical, F.Cu at (116.6, 117.9)
- added J34: Conn_01x02_Pin, Connector_JST:JST_VH_B2P-VH_1x02_P3.96mm_Vertical, F.Cu at (8.70, 118.0)
- added J35: Conn_01x02_Pin, Connector_JST:JST_VH_B2P-VH_1x02_P3.96mm_Vertical, F.Cu at (65.8, 118.1)
- added J36: Conn_01x12_Pin, Connector_JST:JST_ZH_B6B-ZR_1x06_P1.50mm_Vertical, F.Cu at (56.4, 122.6)
- added J37: Conn_01x02_Pin, Connector_JST:JST_VH_B2P-VH_1x02_P3.96mm_Vertical, F.Cu at (116.6, 133.1)
- added J38: Conn_01x02_Pin, Connector_JST:JST_VH_B2P-VH_1x02_P3.96mm_Vertical, F.Cu at (8.70, 133.2)
- added J39: Conn_01x02_Pin, Connector_JST:JST_VH_B2P-VH_1x02_P3.96mm_Vertical, F.Cu at (65.8, 133.3)
- added J40: Conn_01x12_Pin, Connector_JST:JST_ZH_B6B-ZR_1x06_P1.50mm_Vertical, F.Cu at (56.4, 137.9)
- added J41: Conn_01x02_Pin, Connector_JST:JST_VH_B2P-VH_1x02_P3.96mm_Vertical, F.Cu at (8.70, 148.4)
- added J42: Conn_01x02_Pin, Connector_JST:JST_VH_B2P-VH_1x02_P3.96mm_Vertical, F.Cu at (116.6, 148.3)
- added J43: Conn_01x02_Pin, Connector_JST:JST_VH_B2P-VH_1x02_P3.96mm_Vertical, F.Cu at (65.8, 148.5)
- added J44: Conn_01x12_Pin, Connector_JST:JST_ZH_B6B-ZR_1x06_P1.50mm_Vertical, F.Cu at (56.4, 153.1)
- added J45: Conn_01x02_Pin, Connector_JST:JST_VH_B2P-VH_1x02_P3.96mm_Vertical, F.Cu at (8.70, 163.7)
- added J46: Conn_01x02_Pin, Connector_JST:JST_VH_B2P-VH_1x02_P3.96mm_Vertical, F.Cu at (116.6, 163.6)
- added J47: Conn_01x02_Pin, Connector_JST:JST_VH_B2P-VH_1x02_P3.96mm_Vertical, F.Cu at (65.8, 163.8)
- added J48: Conn_01x12_Pin, Connector_JST:JST_ZH_B6B-ZR_1x06_P1.50mm_Vertical, F.Cu at (56.4, 168.3)
- added J49: Conn_01x02_Pin, Connector_JST:JST_VH_B2P-VH_1x02_P3.96mm_Vertical, F.Cu at (116.6, 178.8)
- added J5: Conn_01x02_Pin, Connector_JST:JST_VH_B2P-VH_1x02_P3.96mm_Vertical, F.Cu at (8.70, 11.3)
- added J50: Conn_01x02_Pin, Connector_JST:JST_VH_B2P-VH_1x02_P3.96mm_Vertical, F.Cu at (8.70, 178.9)
- added J51: Conn_01x02_Pin, Connector_JST:JST_VH_B2P-VH_1x02_P3.96mm_Vertical, F.Cu at (65.8, 179.0)
- added J52: Conn_01x12_Pin, Connector_JST:JST_ZH_B6B-ZR_1x06_P1.50mm_Vertical, F.Cu at (56.4, 183.6)
- added J6: Conn_01x02_Pin, Connector_JST:JST_VH_B2P-VH_1x02_P3.96mm_Vertical, F.Cu at (116.6, 11.2)
- added J7: Conn_01x02_Pin, Connector_JST:JST_VH_B2P-VH_1x02_P3.96mm_Vertical, F.Cu at (65.8, 11.4)
- added J8: Conn_01x12_Pin, Connector_JST:JST_ZH_B6B-ZR_1x06_P1.50mm_Vertical, F.Cu at (56.4, 15.9)
- added J9: Conn_01x02_Pin, Connector_JST:JST_VH_B2P-VH_1x02_P3.96mm_Vertical, F.Cu at (116.6, 26.4)
- added L10: ~, Flipdot:Flipdot_single, F.Cu at (15.2, 15.2)
- added L100: ~, Flipdot:Flipdot_single, F.Cu at (45.7, 182.9)
- added L101: ~, Flipdot:Flipdot_single, F.Cu at (61.0, 182.9)
- added L102: ~, Flipdot:Flipdot_single, F.Cu at (76.2, 182.9)
- added L103: ~, Flipdot:Flipdot_single, F.Cu at (91.4, 182.9)
- added L104: ~, Flipdot:Flipdot_single, F.Cu at (106.7, 182.9)
- added L11: ~, Flipdot:Flipdot_single, F.Cu at (30.5, 15.2)
- added L12: ~, Flipdot:Flipdot_single, F.Cu at (45.7, 15.2)
- added L13: ~, Flipdot:Flipdot_single, F.Cu at (61.0, 15.2)
- added L14: ~, Flipdot:Flipdot_single, F.Cu at (76.2, 15.2)
- added L15: ~, Flipdot:Flipdot_single, F.Cu at (91.4, 15.2)
- added L16: ~, Flipdot:Flipdot_single, F.Cu at (106.7, 15.2)
- added L17: ~, Flipdot:Flipdot_single, F.Cu at (0.00, 30.5)
- added L18: ~, Flipdot:Flipdot_single, F.Cu at (15.2, 30.5)
- added L19: ~, Flipdot:Flipdot_single, F.Cu at (30.5, 30.5)
- added L20: ~, Flipdot:Flipdot_single, F.Cu at (45.7, 30.5)
- added L21: ~, Flipdot:Flipdot_single, F.Cu at (61.0, 30.5)
- added L22: ~, Flipdot:Flipdot_single, F.Cu at (76.2, 30.5)
- added L23: ~, Flipdot:Flipdot_single, F.Cu at (91.4, 30.5)
- added L24: ~, Flipdot:Flipdot_single, F.Cu at (106.7, 30.5)
- added L25: ~, Flipdot:Flipdot_single, F.Cu at (0.00, 45.7)
- added L26: ~, Flipdot:Flipdot_single, F.Cu at (15.2, 45.7)
- added L27: ~, Flipdot:Flipdot_single, F.Cu at (30.5, 45.7)
- added L28: ~, Flipdot:Flipdot_single, F.Cu at (45.7, 45.7)
- added L29: ~, Flipdot:Flipdot_single, F.Cu at (61.0, 45.7)
- added L30: ~, Flipdot:Flipdot_single, F.Cu at (76.2, 45.7)
- added L31: ~, Flipdot:Flipdot_single, F.Cu at (91.4, 45.7)
- added L32: ~, Flipdot:Flipdot_single, F.Cu at (106.7, 45.7)
- added L33: ~, Flipdot:Flipdot_single, F.Cu at (0.00, 61.0)
- added L34: ~, Flipdot:Flipdot_single, F.Cu at (15.2, 61.0)
- added L35: ~, Flipdot:Flipdot_single, F.Cu at (30.5, 61.0)
- added L36: ~, Flipdot:Flipdot_single, F.Cu at (45.7, 61.0)
- added L37: ~, Flipdot:Flipdot_single, F.Cu at (61.0, 61.0)
- added L38: ~, Flipdot:Flipdot_single, F.Cu at (76.2, 61.0)
- added L39: ~, Flipdot:Flipdot_single, F.Cu at (91.4, 61.0)
- added L40: ~, Flipdot:Flipdot_single, F.Cu at (106.7, 61.0)
- added L41: ~, Flipdot:Flipdot_single, F.Cu at (0.00, 76.2)
- added L42: ~, Flipdot:Flipdot_single, F.Cu at (15.2, 76.2)
- added L43: ~, Flipdot:Flipdot_single, F.Cu at (30.5, 76.2)
- added L44: ~, Flipdot:Flipdot_single, F.Cu at (45.7, 76.2)
- added L45: ~, Flipdot:Flipdot_single, F.Cu at (61.0, 76.2)
- added L46: ~, Flipdot:Flipdot_single, F.Cu at (76.2, 76.2)
- added L47: ~, Flipdot:Flipdot_single, F.Cu at (91.4, 76.2)
- added L48: ~, Flipdot:Flipdot_single, F.Cu at (106.7, 76.2)
- added L49: ~, Flipdot:Flipdot_single, F.Cu at (0.00, 91.4)
- added L50: ~, Flipdot:Flipdot_single, F.Cu at (15.2, 91.4)
- added L51: ~, Flipdot:Flipdot_single, F.Cu at (30.5, 91.4)
- added L52: ~, Flipdot:Flipdot_single, F.Cu at (45.7, 91.4)
- added L53: ~, Flipdot:Flipdot_single, F.Cu at (61.0, 91.4)
- added L54: ~, Flipdot:Flipdot_single, F.Cu at (76.2, 91.4)
- added L55: ~, Flipdot:Flipdot_single, F.Cu at (91.4, 91.4)
- added L56: ~, Flipdot:Flipdot_single, F.Cu at (106.7, 91.4)
- added L57: ~, Flipdot:Flipdot_single, F.Cu at (0.00, 106.7)
- added L58: ~, Flipdot:Flipdot_single, F.Cu at (15.2, 106.7)
- added L59: ~, Flipdot:Flipdot_single, F.Cu at (30.5, 106.7)
- added L60: ~, Flipdot:Flipdot_single, F.Cu at (45.7, 106.7)
- added L61: ~, Flipdot:Flipdot_single, F.Cu at (61.0, 106.7)
- added L62: ~, Flipdot:Flipdot_single, F.Cu at (76.2, 106.7)
- added L63: ~, Flipdot:Flipdot_single, F.Cu at (91.4, 106.7)
- added L64: ~, Flipdot:Flipdot_single, F.Cu at (106.7, 106.7)
- added L65: ~, Flipdot:Flipdot_single, F.Cu at (0.00, 121.9)
- added L66: ~, Flipdot:Flipdot_single, F.Cu at (15.2, 121.9)
- added L67: ~, Flipdot:Flipdot_single, F.Cu at (30.5, 121.9)
- added L68: ~, Flipdot:Flipdot_single, F.Cu at (45.7, 121.9)
- added L69: ~, Flipdot:Flipdot_single, F.Cu at (61.0, 121.9)
- added L70: ~, Flipdot:Flipdot_single, F.Cu at (76.2, 121.9)
- added L71: ~, Flipdot:Flipdot_single, F.Cu at (91.4, 121.9)
- added L72: ~, Flipdot:Flipdot_single, F.Cu at (106.7, 121.9)
- added L73: ~, Flipdot:Flipdot_single, F.Cu at (0.00, 137.2)
- added L74: ~, Flipdot:Flipdot_single, F.Cu at (15.2, 137.2)
- added L75: ~, Flipdot:Flipdot_single, F.Cu at (30.5, 137.2)
- added L76: ~, Flipdot:Flipdot_single, F.Cu at (45.7, 137.2)
- added L77: ~, Flipdot:Flipdot_single, F.Cu at (61.0, 137.2)
- added L78: ~, Flipdot:Flipdot_single, F.Cu at (76.2, 137.2)
- added L79: ~, Flipdot:Flipdot_single, F.Cu at (91.4, 137.2)
- added L80: ~, Flipdot:Flipdot_single, F.Cu at (106.7, 137.2)
- added L81: ~, Flipdot:Flipdot_single, F.Cu at (0.00, 152.4)
- added L82: ~, Flipdot:Flipdot_single, F.Cu at (15.2, 152.4)
- added L83: ~, Flipdot:Flipdot_single, F.Cu at (30.5, 152.4)
- added L84: ~, Flipdot:Flipdot_single, F.Cu at (45.7, 152.4)
- added L85: ~, Flipdot:Flipdot_single, F.Cu at (61.0, 152.4)
- added L86: ~, Flipdot:Flipdot_single, F.Cu at (76.2, 152.4)
- added L87: ~, Flipdot:Flipdot_single, F.Cu at (91.4, 152.4)
- added L88: ~, Flipdot:Flipdot_single, F.Cu at (106.7, 152.4)
- added L89: ~, Flipdot:Flipdot_single, F.Cu at (0.00, 167.6)
- added L9: ~, Flipdot:Flipdot_single, F.Cu at (0.00, 15.2)
- added L90: ~, Flipdot:Flipdot_single, F.Cu at (15.2, 167.6)
- added L91: ~, Flipdot:Flipdot_single, F.Cu at (30.5, 167.6)
- added L92: ~, Flipdot:Flipdot_single, F.Cu at (45.7, 167.6)
- added L93: ~, Flipdot:Flipdot_single, F.Cu at (61.0, 167.6)
- added L94: ~, Flipdot:Flipdot_single, F.Cu at (76.2, 167.6)
- added L95: ~, Flipdot:Flipdot_single, F.Cu at (91.4, 167.6)
- added L96: ~, Flipdot:Flipdot_single, F.Cu at (106.7, 167.6)
- added L97: ~, Flipdot:Flipdot_single, F.Cu at (0.00, 182.9)
- added L98: ~, Flipdot:Flipdot_single, F.Cu at (15.2, 182.9)
- added L99: ~, Flipdot:Flipdot_single, F.Cu at (30.5, 182.9)
- added U10: ~, Package_SO:SOP-8_3.9x4.9mm_P1.27mm, F.Cu at (15.6, 7.34)
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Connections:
- net /row1/CLK renamed CLK
- net /row1/LATCH renamed LATCH
- net /row1/OE* renamed OE*
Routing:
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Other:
- board size 121.3 x 14.6 mm -> 121.3 x 197.5 mm
